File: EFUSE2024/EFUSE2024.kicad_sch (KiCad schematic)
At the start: 22 parts, among them Q3 CSD19532Q5B, Q4 CSD19532Q5B, Q7 BSS138, U5 TPS26631PWP, U6 TPS26631PWP, U7 TPS26630RGE

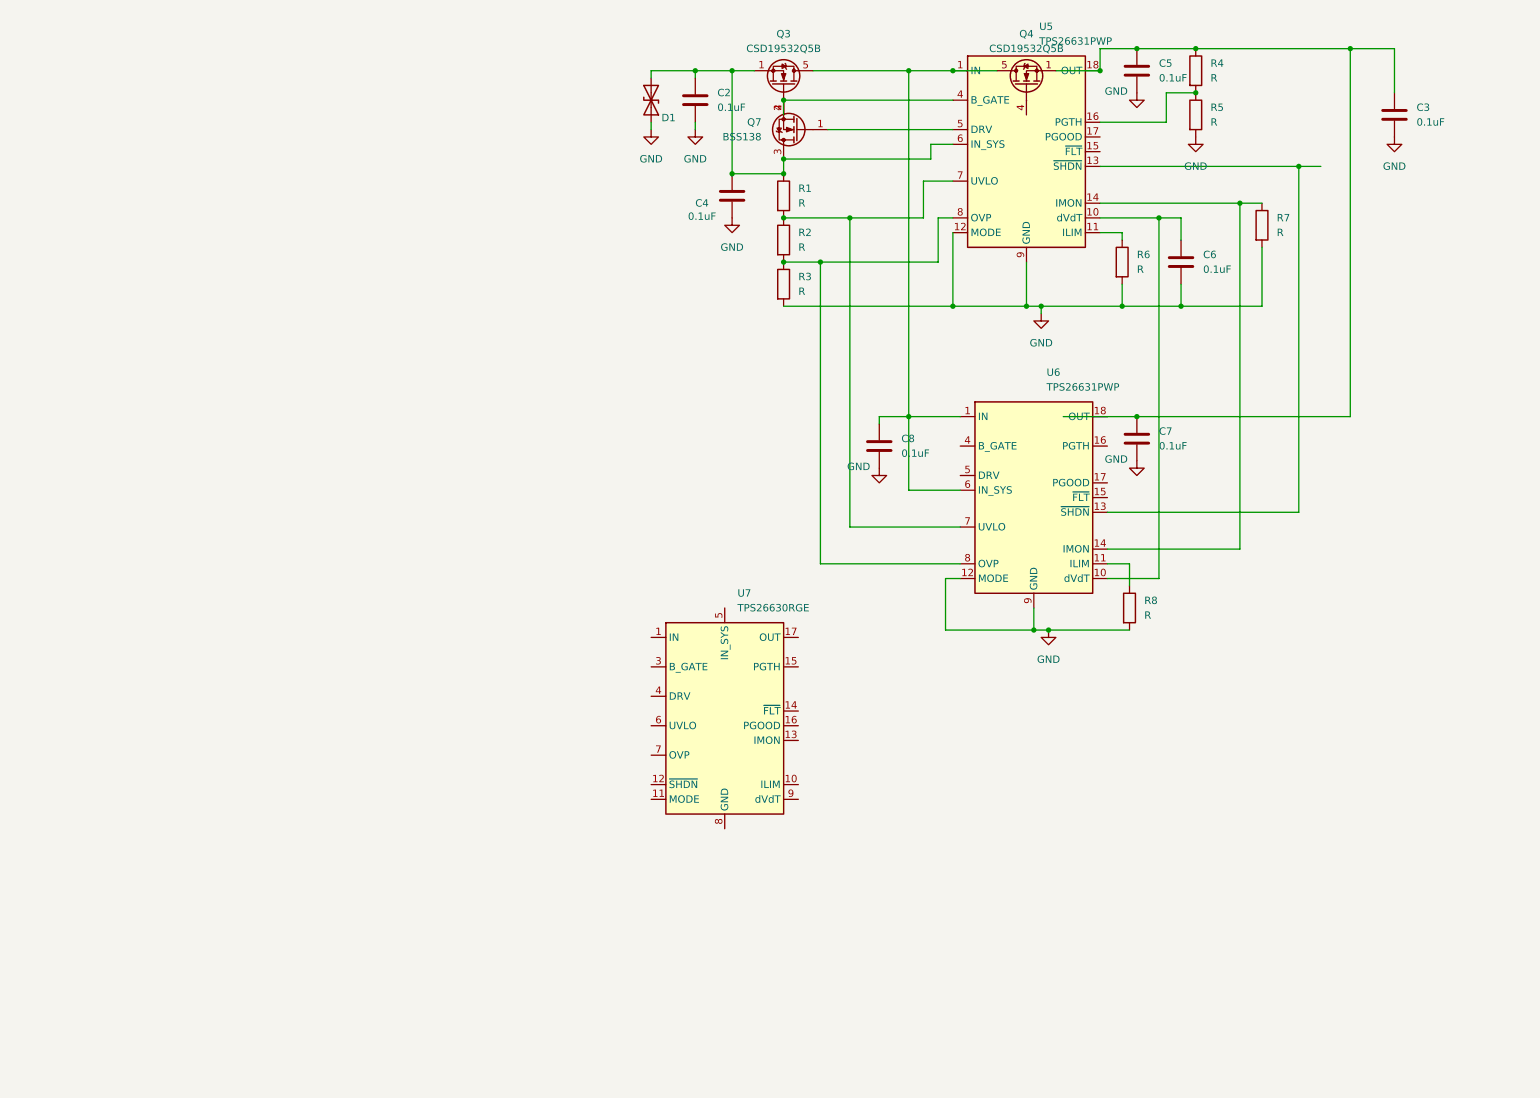
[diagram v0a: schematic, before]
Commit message: schematic
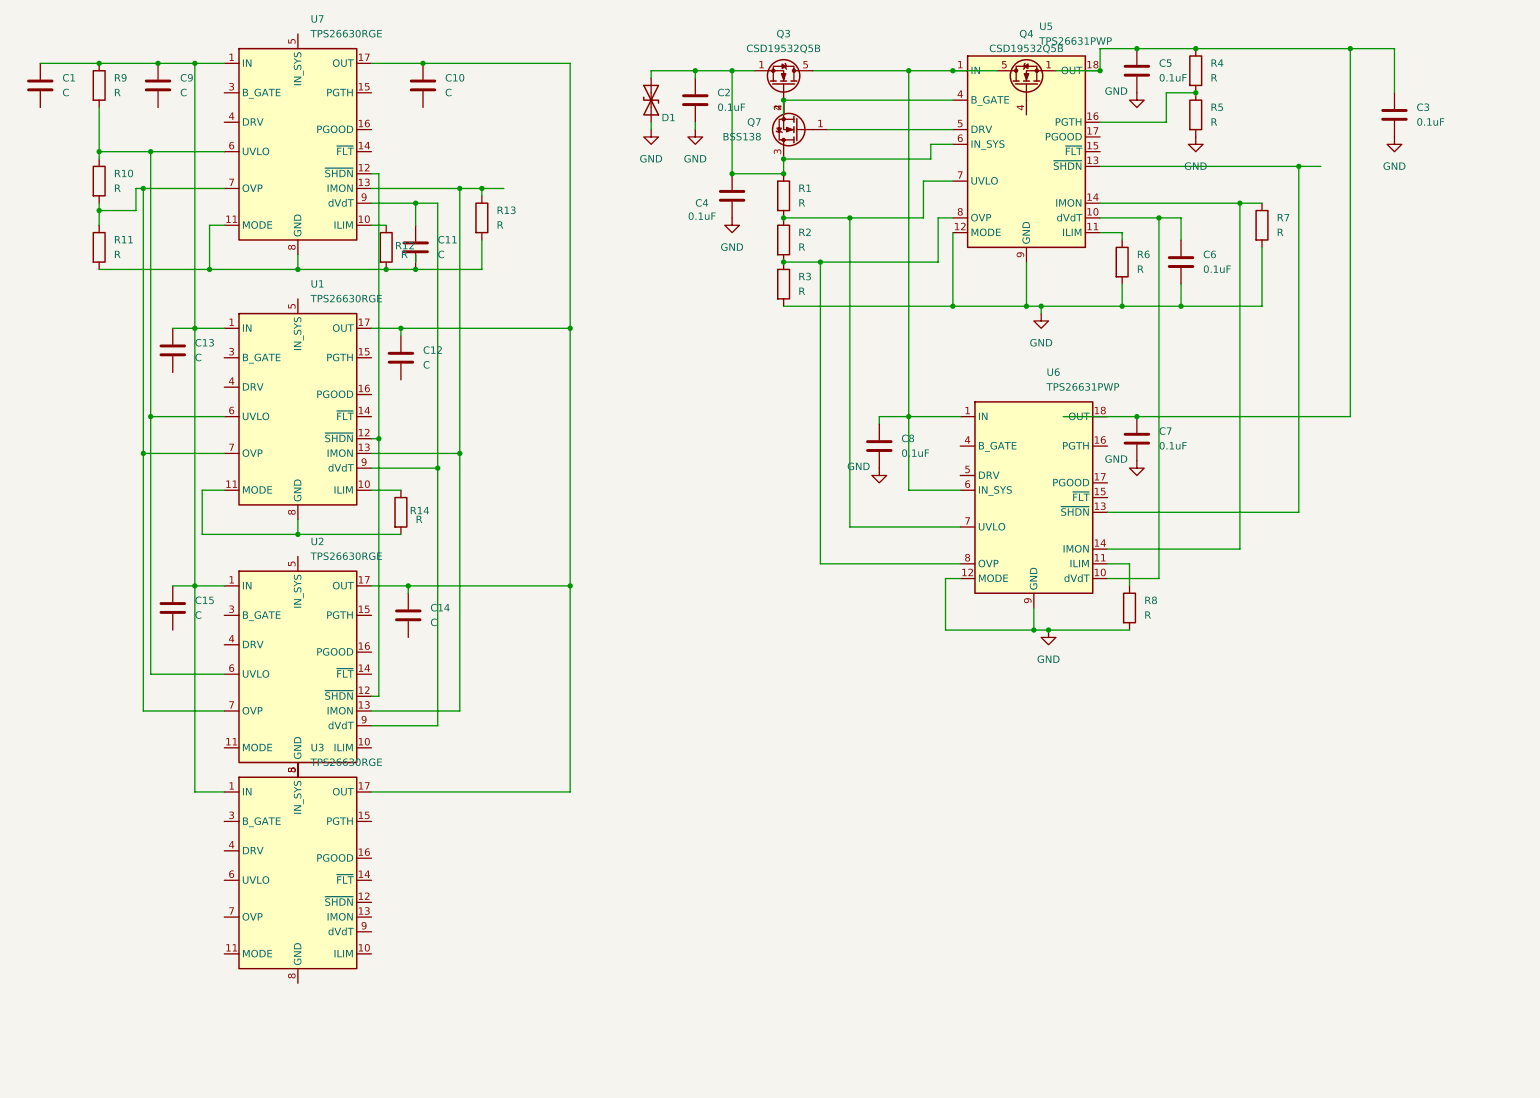
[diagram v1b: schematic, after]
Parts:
- added C1, C10, C11, C12, C13, C14, C15, C9: C, symbol Device:C
- added R10, R11, R12, R13, R14, R9: R, symbol Device:R
- added U1, U2, U3: TPS26630RGE, Package_DFN_QFN:Texas_RGE0024H_VQFN-24-1EP_4x4mm_P0.5mm_EP2.7x2.7mm_ThermalVias, symbol Power_Management:TPS26630RGE
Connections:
- net at U7.1 (IN), U7.2 (IN): now also C1.1, C13.1, C15.1, C9.1, R9.1, U1.1 (IN), U1.2 (IN), U2.1 (IN), U2.2 (IN), U3.1 (IN), U3.2 (IN)
- net at U7.10 (ILIM): now also R12.1
- net at U7.11 (MODE): now also U7.25 (GND), U7.8 (GND), C11.2, R11.2, R12.2, R13.2
- net at U7.12 (~{SHDN}): now also U1.12 (~{SHDN}), U2.12 (~{SHDN})
- net at U7.13 (IMON): now also R13.1, U1.13 (IMON), U2.13 (IMON)
- net at U7.17 (OUT), U7.18 (OUT): now also C10.1, C12.1, C14.1, U1.17 (OUT), U1.18 (OUT), U2.17 (OUT), U2.18 (OUT), U3.17 (OUT), U3.18 (OUT)
- net at U7.6 (UVLO): now also R10.1, R9.2, U1.6 (UVLO), U2.6 (UVLO)
- net at U7.7 (OVP): now also R10.2, R11.1, U1.7 (OVP), U2.7 (OVP)
- net at U7.9 (dVdT): now also C11.1, U1.9 (dVdT), U2.9 (dVdT)
- new net: U3.25 (GND), U3.8 (GND)
- new net: R14.1, U1.10 (ILIM)
- new net: R14.2, U1.11 (MODE), U1.25 (GND), U1.8 (GND)
- new net: U2.25 (GND), U2.8 (GND)
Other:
- moved on the sheet: U7

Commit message: Adding to schematic
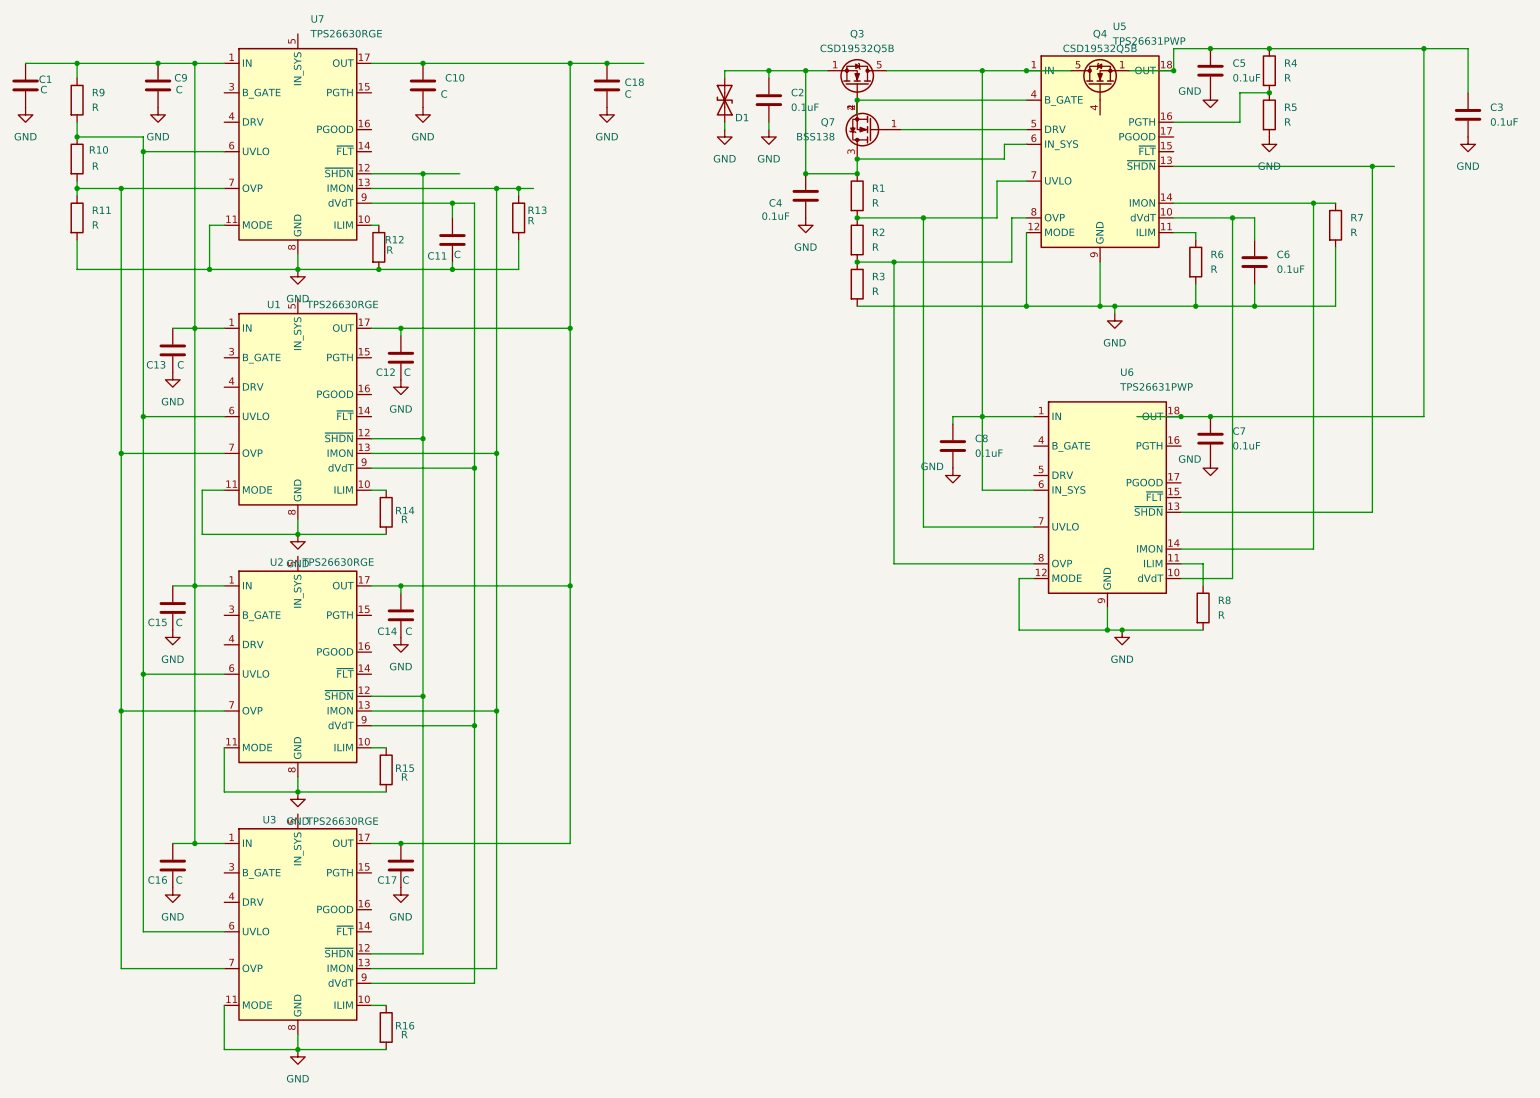
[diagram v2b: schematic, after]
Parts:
- added C16, C17, C18: C, symbol Device:C
- added R15, R16: R, symbol Device:R
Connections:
- net GND: now also C1.2, C10.2, C11.2, C12.2, C13.2, C14.2, C15.2, C9.2, R11.2, R12.2, R13.2, R14.2, U1.11 (MODE), U1.25 (GND), U1.8 (GND), U2.11 (MODE), U2.25 (GND), U2.8 (GND), U3.11 (MODE), U3.25 (GND), U3.8 (GND), U7.11 (MODE), U7.25 (GND), U7.8 (GND), C16.2, C17.2, C18.2, R15.2, R16.2
- net at C1.1, C13.1, C15.1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: now also C16.1
- net at U1.12 (~{SHDN}), U2.12 (~{SHDN}), U7.12 (~{SHDN}): now also U3.12 (~{SHDN})
- net at R13.1, U1.13 (IMON), U2.13 (IMON)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: now also U3.13 (IMON)
- net at C10.1, C12.1, C14.1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: now also C17.1, C18.1
- net at R10.1, R9.2, U1.6 (UVLO)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: now also U3.6 (UVLO)
- net at R10.2, R11.1, U1.7 (OVP)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: now also U3.7 (OVP)
- net at C11.1, U1.9 (dVdT), U2.9 (dVdT)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: now also U3.9 (dVdT)
- net at U3.10 (ILIM): now also R16.1
- net at U2.10 (ILIM): now also R15.1
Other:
- moved on the sheet: C1, C11, C14, C2, C3, C4, C5, C6, C7, C8, D1, Q3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
